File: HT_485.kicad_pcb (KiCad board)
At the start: 2 copper layers, 82 x 72.2 mm, 85 parts, among them J1 POWER, J2 485, J3 PT1000, J4 H/T Sensor, J5 PRG, Q1 BC817, Q2 BC817, Q3 BC817, Q4 BC817, U1 MAX14786EAUD+T, U2 TL082, U3 LM2576D2TR4-3.3G, U4 ESP32-S3-WROOM-1-N16R8, U5 CAT3200TDI-GT3, U6 L7815

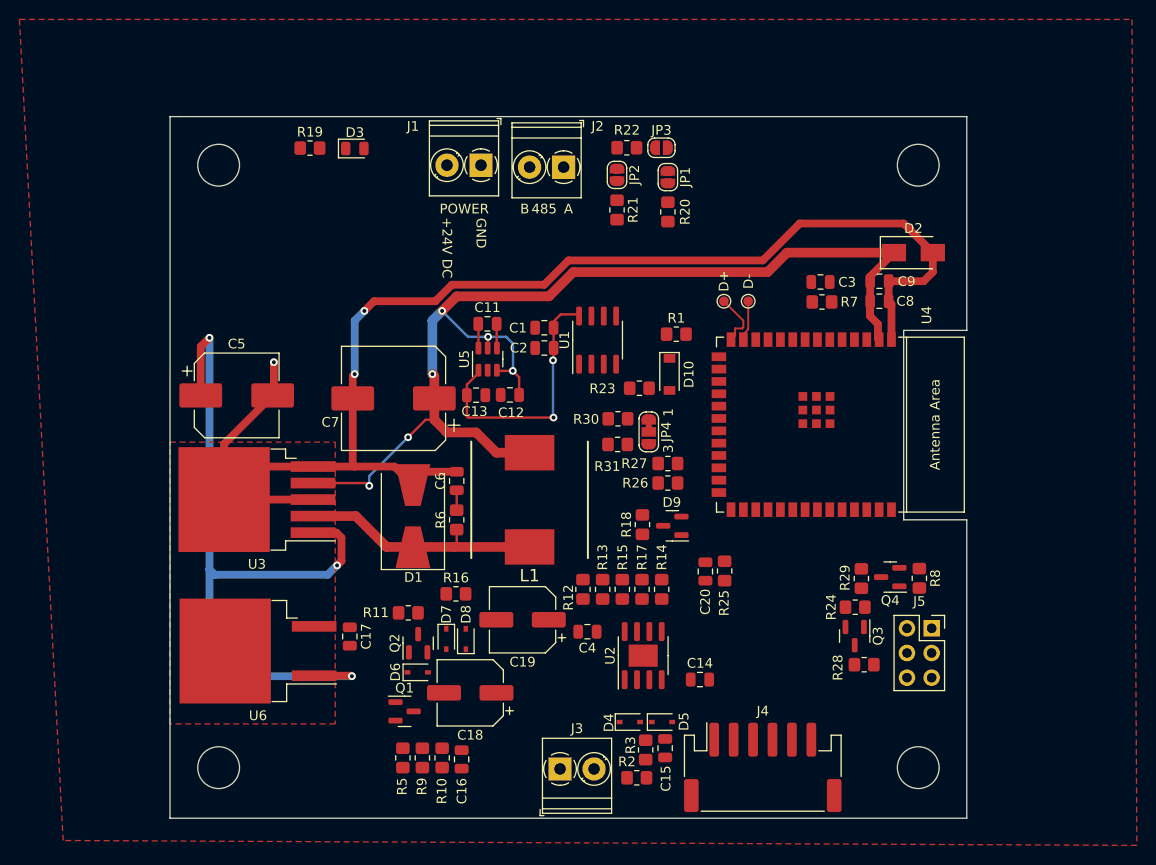
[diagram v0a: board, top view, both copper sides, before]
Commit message: Rifatto schema 485. Master da rifare
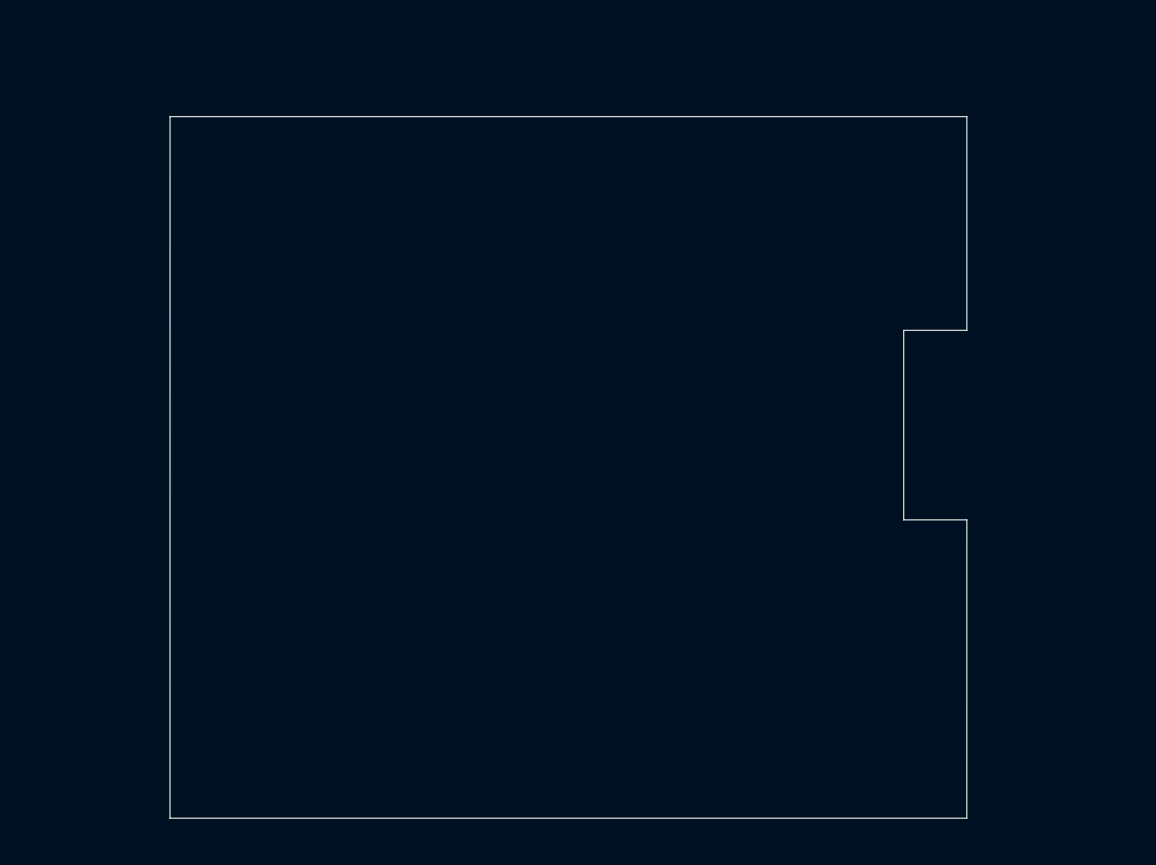
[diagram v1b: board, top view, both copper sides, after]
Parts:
- removed C1: 4.7uF, Capacitor_SMD:C_0805_2012Metric
- removed C11, C12: 1uF, Capacitor_SMD:C_0805_2012Metric
- removed C13, C9: 10uF, Capacitor_SMD:C_0805_2012Metric
- removed C14, C15, C2, C20, C4, C8: 100nF, Capacitor_SMD:C_0805_2012Metric
- removed C16: 1nF, Capacitor_SMD:C_0805_2012Metric
- removed C17: 1uF/25V, Capacitor_SMD:C_0805_2012Metric
- removed C18, C19: 100uF/25V, Capacitor_SMD:CP_Elec_6.3x7.7
- removed C3: 1uF/16V, Capacitor_SMD:C_0805_2012Metric
- removed C5: 100uF / 50V, Capacitor_SMD:CP_Elec_8x10.5
- removed C6: 1nF/10V, Capacitor_SMD:C_0805_2012Metric
- removed C7: 1000uF/10V, Capacitor_SMD:CP_Elec_10x10.5
- removed D1: VS-30BQ060HM3/9AT, Diode_SMD:D_SMB-SMC_Universal_Handsoldering
- removed D10: STPS0520Z, Diode_SMD:D_SOD-123
- removed D2: 3.9V/1W, Diode_SMD:D_SMA
- removed D3: PWR, LED_SMD:LED_0805_2012Metric
- removed D4, D5, D6, D7, D8: 1N4148WS, Diode_SMD:D_SOD-323
- removed D9: BAV99, Package_TO_SOT_SMD:SOT-23
- removed J1: POWER, TerminalBlock_Phoenix:TerminalBlock_Phoenix_PT-1,5-2-3.5-H_1x02_P3.50mm_Horizontal
- removed J2: 485, TerminalBlock_Phoenix:TerminalBlock_Phoenix_PT-1,5-2-3.5-H_1x02_P3.50mm_Horizontal
- removed J3: PT1000, TerminalBlock_Phoenix:TerminalBlock_Phoenix_PT-1,5-2-3.5-H_1x02_P3.50mm_Horizontal
- removed J4: H/T Sensor, Connector_JST:JST_PH_S6B-PH-SM4-TB_1x06-1MP_P2.00mm_Horizontal
- removed J5: PRG, Connector_PinSocket_2.54mm:PinSocket_2x03_P2.54mm_Vertical
- removed JP1: BIAS+, Jumper:SolderJumper-2_P1.3mm_Open_RoundedPad1.0x1.5mm
- removed JP2: BIAS-, Jumper:SolderJumper-2_P1.3mm_Open_RoundedPad1.0x1.5mm
- removed JP3: TERMINATOR, Jumper:SolderJumper-2_P1.3mm_Open_RoundedPad1.0x1.5mm
- removed JP4: UART_BOOT_MSG, Jumper:SolderJumper-3_P1.3mm_Bridged12_RoundedPad1.0x1.5mm_NumberLabels
- removed L1: 100uH -MSS1210-104KED, HT485:MSS1210-104KED
- removed Q1, Q2, Q3, Q4: BC817, Package_TO_SOT_SMD:SOT-23
- removed R1, R11, R14, R18, R19, R24, R25, R26, R27, R3, R30, R31, R5, R7, R8: 10K, Resistor_SMD:R_0805_2012Metric_Pad1.20x1.40mm_HandSolder
- removed R10: 100R, Resistor_SMD:R_0805_2012Metric_Pad1.20x1.40mm_HandSolder
- removed R12, R13, R15, R9: 1K, Resistor_SMD:R_0805_2012Metric_Pad1.20x1.40mm_HandSolder
- removed R16, R6: 10R, Resistor_SMD:R_0805_2012Metric_Pad1.20x1.40mm_HandSolder
- removed R17: 3k3, Resistor_SMD:R_0805_2012Metric_Pad1.20x1.40mm_HandSolder
- removed R2: 1K 1%, Resistor_SMD:R_0805_2012Metric_Pad1.20x1.40mm_HandSolder
- removed R20, R21: 370R, Resistor_SMD:R_0805_2012Metric_Pad1.20x1.40mm_HandSolder
- removed R22: 120R, Resistor_SMD:R_0805_2012Metric_Pad1.20x1.40mm_HandSolder
- removed R23: 4K7, Resistor_SMD:R_0805_2012Metric_Pad1.20x1.40mm_HandSolder
- removed R28, R29: 0R, Resistor_SMD:R_0805_2012Metric_Pad1.20x1.40mm_HandSolder
- removed REF** (x4): MountingHole_4.3mm_M4, MountingHole:MountingHole_4.3mm_M4
- removed TP1: D+, TestPoint:TestPoint_Pad_D1.0mm
- removed TP2: D-, TestPoint:TestPoint_Pad_D1.0mm
- removed U1: MAX14786EAUD+T, Package_SO:SOIC-8_3.9x4.9mm_P1.27mm
- removed U2: TL082, Package_SO:SOIC-8-1EP_3.9x4.9mm_P1.27mm_EP2.29x3mm
- removed U3: LM2576D2TR4-3.3G, Package_TO_SOT_SMD:TO-263-5_TabPin3
- removed U4: ESP32-S3-WROOM-1-N16R8, Espressif:ESP32-S3-WROOM-1
- removed U5: CAT3200TDI-GT3, Package_TO_SOT_SMD:TSOT-23-6
- removed U6: L7815, Package_TO_SOT_SMD:TO-263-2
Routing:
- net GND: track 145.7 -> 0.00 mm, vias 3 -> 0
- net +3V3: track 117.3 -> 0.00 mm, vias 6 -> 0
- net +24V: track 79.0 -> 0.00 mm, vias 3 -> 0
- net +5V: track 27.1 -> 0.00 mm, vias 2 -> 0
- net Net-(D1-Pad1): track 25.5 -> 0.00 mm
- net /D+: track 5.73 -> 0.00 mm
- net /D-: track 4.16 -> 0.00 mm
- net Net-(C11-Pad1): track 2.51 -> 0.00 mm
- net Net-(C11-Pad2): track 2.51 -> 0.00 mm
- net Net-(C6-Pad1): track 2.05 -> 0.00 mm
- removed copper zone on F.Cu, net GND
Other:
- board text removed: "${COMPANY} ${TITLE} V: ${REVISION} DATE: ${ISSUE_DATE} ${COMMENT1}"
- board text removed: "+24V DC"
- board text removed: "A"
- board text removed: "B"
- board text removed: "GND"
